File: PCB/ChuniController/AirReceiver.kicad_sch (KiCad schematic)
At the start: 3 parts, among them J7 Conn_01x08

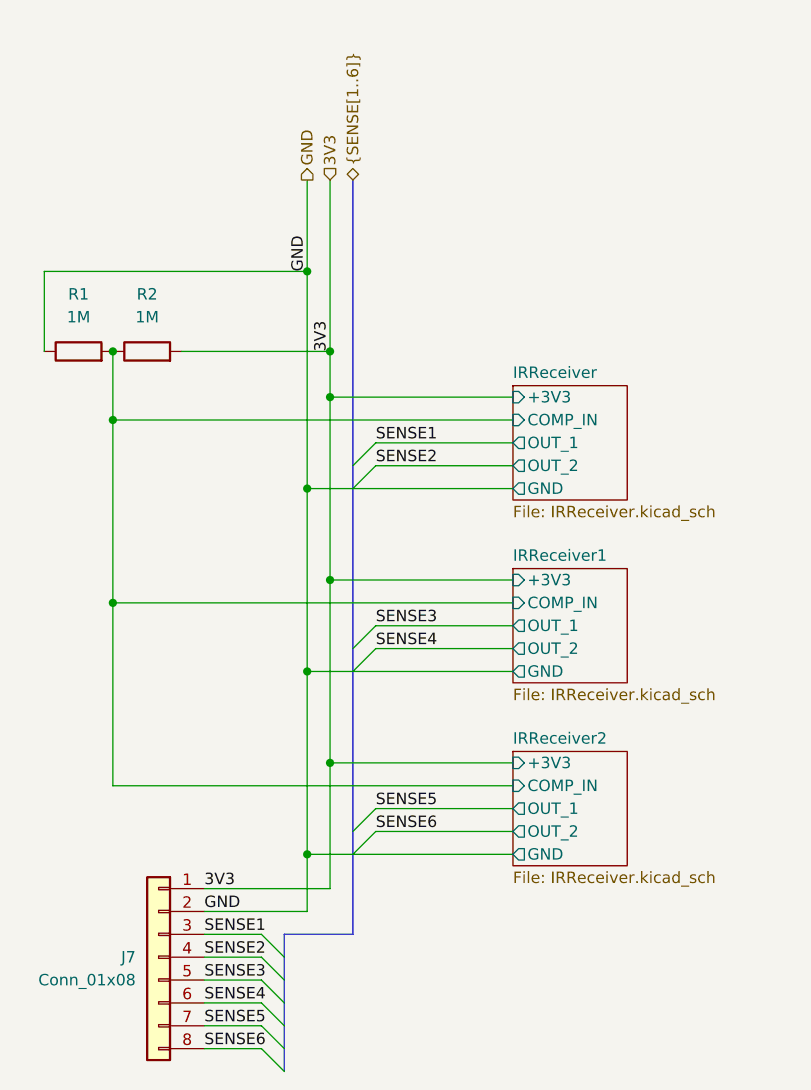
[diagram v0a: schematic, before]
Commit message: PCB
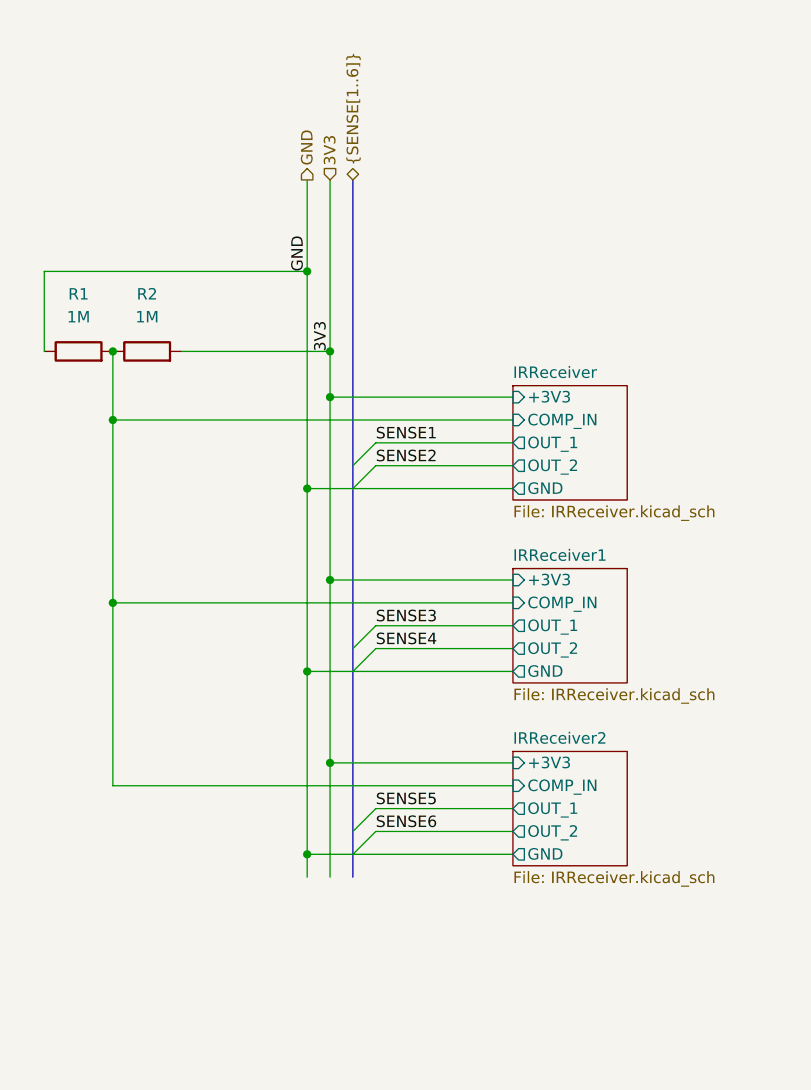
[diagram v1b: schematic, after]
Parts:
- removed J7: Conn_01x08, Connector_JST:JST_SH_SM08B-SRSS-TB_1x08-1MP_P1.00mm_Horizontal, symbol Connector_Generic:Conn_01x08
